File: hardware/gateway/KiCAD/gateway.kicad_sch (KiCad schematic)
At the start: 18 parts, among them J1 USB-C input, J2 Buzzer, Q1 AO3400A, SW1 SW_Push, U1 ESP32-C3_SUPERMINI_TH, U2 Ai-Thinker-Ra-02, U3 AMS1117-3.3

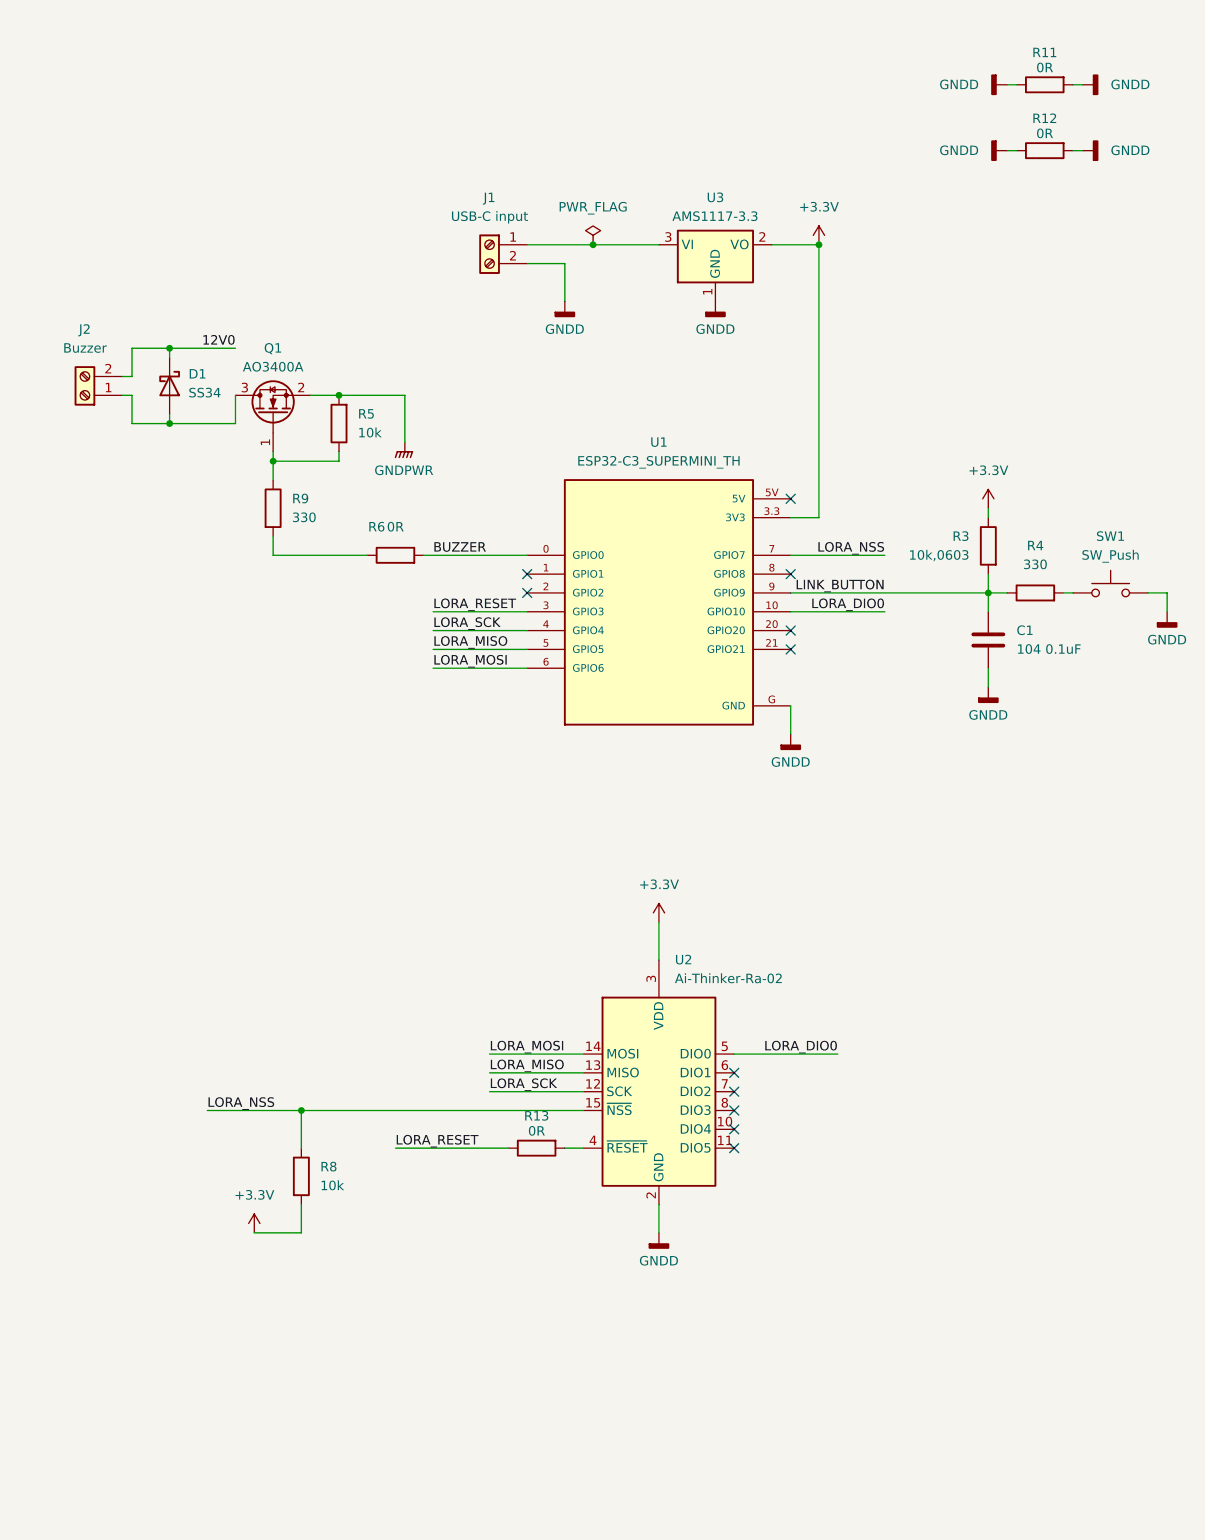
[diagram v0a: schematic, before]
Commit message: dev
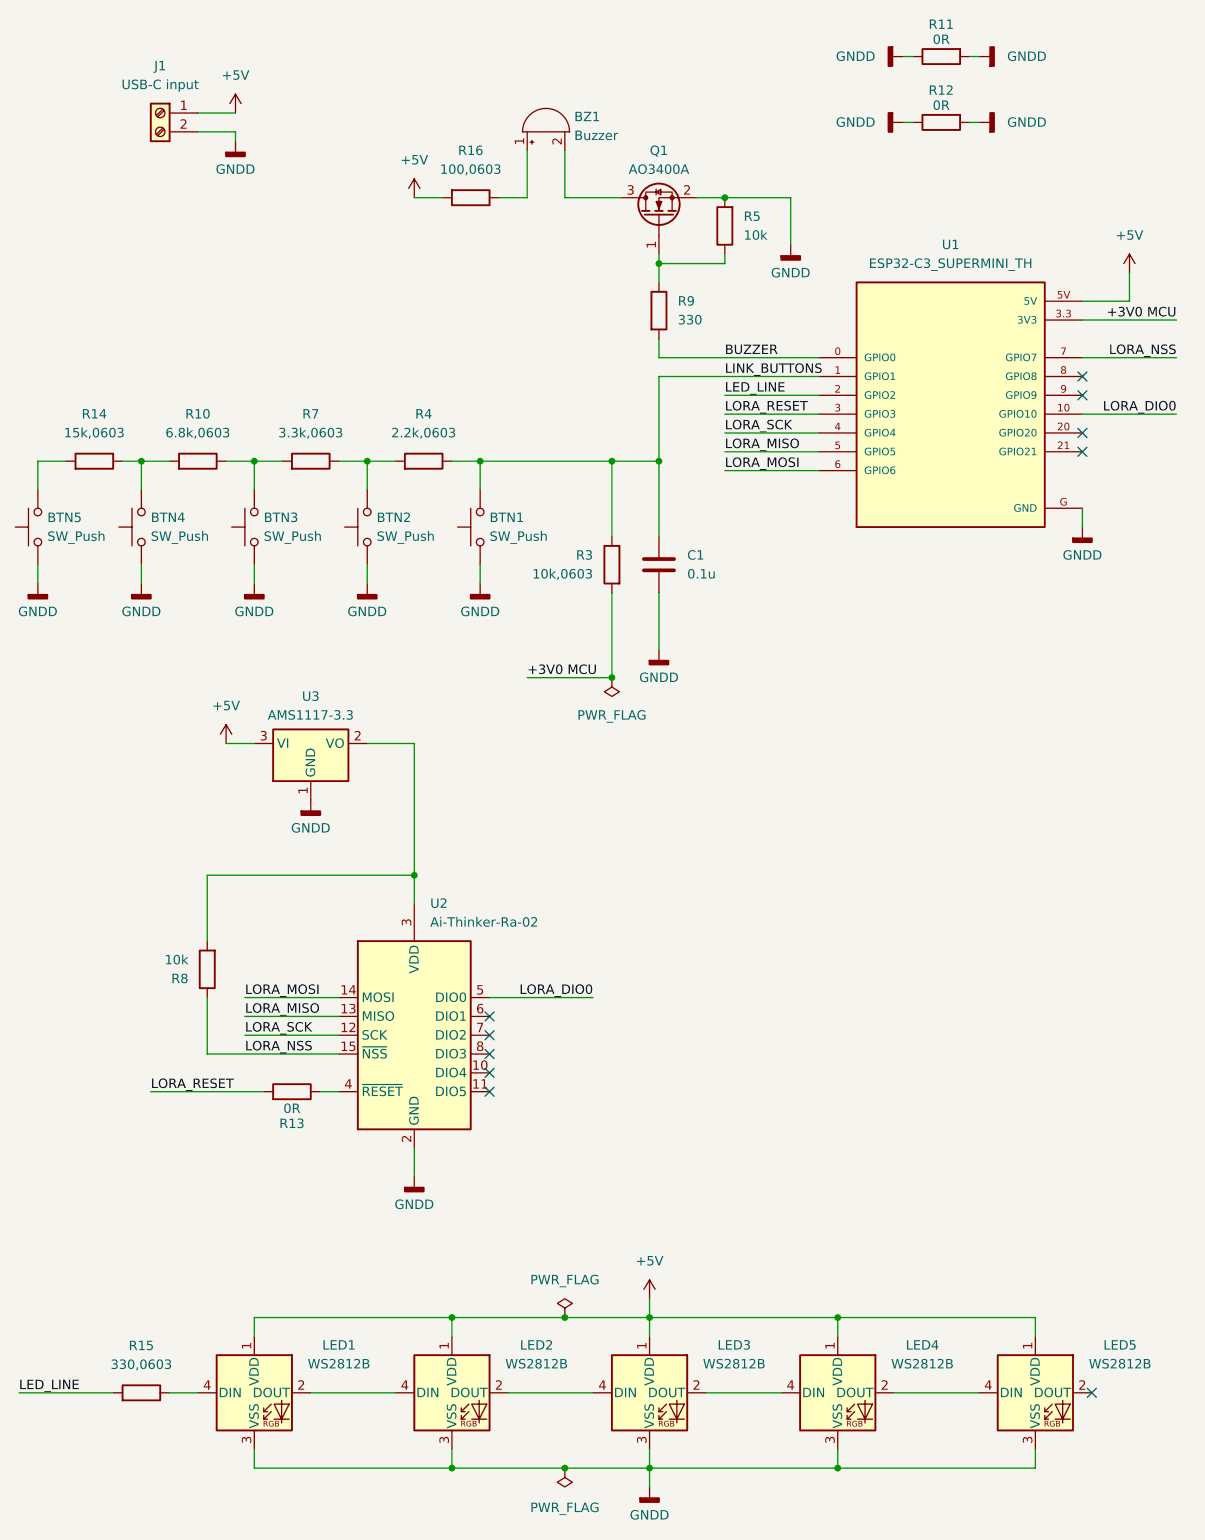
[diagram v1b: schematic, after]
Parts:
- removed D1: SS34, Diode_SMD:D_SMA, symbol Diode:SS34
- removed J2: Buzzer, TerminalBlock_Phoenix:TerminalBlock_Phoenix_MKDS-1,5-2_1x02_P5.00mm_Horizontal, symbol Connector:Screw_Terminal_01x02
- removed R6: 0R, Resistor_SMD:R_2512_6332Metric_Pad1.40x3.35mm_HandSolder, symbol Device:R
- removed SW1: SW_Push, Button_Switch_THT:SW_PUSH_6mm_H5mm, symbol Switch:SW_Push
- added BTN1, BTN2, BTN3, BTN4, BTN5: SW_Push, Button_Switch_THT:SW_PUSH_6mm_H5mm, symbol Switch:SW_Push
- added BZ1: Buzzer, Buzzer_Beeper:Buzzer_12x9.5RM7.6, symbol Device:Buzzer
- added LED1, LED2, LED3, LED4, LED5: WS2812B, LED_SMD:LED_WS2812B_PLCC4_5.0x5.0mm_P3.2mm, symbol LED:WS2812B
- added R10: 6.8k,0603, Resistor_SMD:R_1206_3216Metric_Pad1.30x1.75mm_HandSolder, symbol Device:R
- added R14: 15k,0603, Resistor_SMD:R_1206_3216Metric_Pad1.30x1.75mm_HandSolder, symbol Device:R
- added R15: 330,0603, Resistor_SMD:R_1206_3216Metric_Pad1.30x1.75mm_HandSolder, symbol Device:R
- added R16: 100,0603, Resistor_SMD:R_1206_3216Metric_Pad1.30x1.75mm_HandSolder, symbol Device:R
- added R7: 3.3k,0603, Resistor_SMD:R_1206_3216Metric_Pad1.30x1.75mm_HandSolder, symbol Device:R
- C1: value 104 0.1uF -> 0.1u
- R4: value 330 -> 2.2k,0603
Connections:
- net GNDPWR is gone; now on net GNDD: Q1.2 (S), R5.2
- net BUZZER: now also R9.2
- net GNDD: now also BTN1.1, BTN2.1, BTN3.1, BTN4.1, BTN5.1, LED1.3 (VSS), LED2.3 (VSS), LED3.3 (VSS), LED4.3 (VSS), LED5.3 (VSS)
- net LORA_RESET: now also R13.2; no longer R13.1
- net +5V: now reaches J1.1 (Pin_1), U3.3 (VI)
- net +5V: now also U1.5V, LED1.1 (VDD), LED2.1 (VDD), LED3.1 (VDD), LED4.1 (VDD), LED5.1 (VDD), R16.2
- net at R4.2: now also BTN2.2, R7.1
- net at U2.4 (~{RESET}): now also R13.1; no longer R13.2
- net LINK_BUTTONS: now reaches U1.1 (GPIO1)
- net LINK_BUTTONS: now also C1.1, R3.1, R4.1, BTN1.2
- net LED_LINE: now reaches U1.2 (GPIO2)
- net LED_LINE: now also R15.2
- net at Q1.3 (D): now also BZ1.2 (-)
- net +3.3V: no longer names the net of R8.2, U2.3 (VDD), U3.2 (VO)
- net +3.3V: no longer R3.1, U1.3.3 (3V3)
- removed net LINK_BUTTON: C1.1, R3.2, R4.1, U1.9 (GPIO9)
- new net: LED3.2 (DOUT), LED4.4 (DIN)
- new net: LED2.2 (DOUT), LED3.4 (DIN)
- new net: LED4.2 (DOUT), LED5.4 (DIN)
- new net: BTN3.2, R10.1, R7.2
- new net: BZ1.1 (+), R16.1
- new net: LED1.2 (DOUT), LED2.4 (DIN)
- new net: BTN4.2, R10.2, R14.1
- new net: LED1.4 (DIN), R15.1
- new net: BTN5.2, R14.2
- new net +3V0 MCU: R3.2, U1.3.3 (3V3)
- no-connect marks 11 -> 10
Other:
- moved on the sheet: J1, Q1, R11, R12, R13, R5, R8, R9, U1, U2, U3
